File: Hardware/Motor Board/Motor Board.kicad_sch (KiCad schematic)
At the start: 14 parts, among them J1 Screw_Terminal_01x03, J2 DIN-5, J3 Conn_02x06_Counter_Clockwise, J4 Screw_Terminal_01x02, J5 Screw_Terminal_01x04, J6 Screw_Terminal_01x05, K1 SRD-24VDC-SL-C, K2 SRD-24VDC-SL-C, K3 SRD-24VDC-SL-C, K4 SRD-24VDC-SL-C

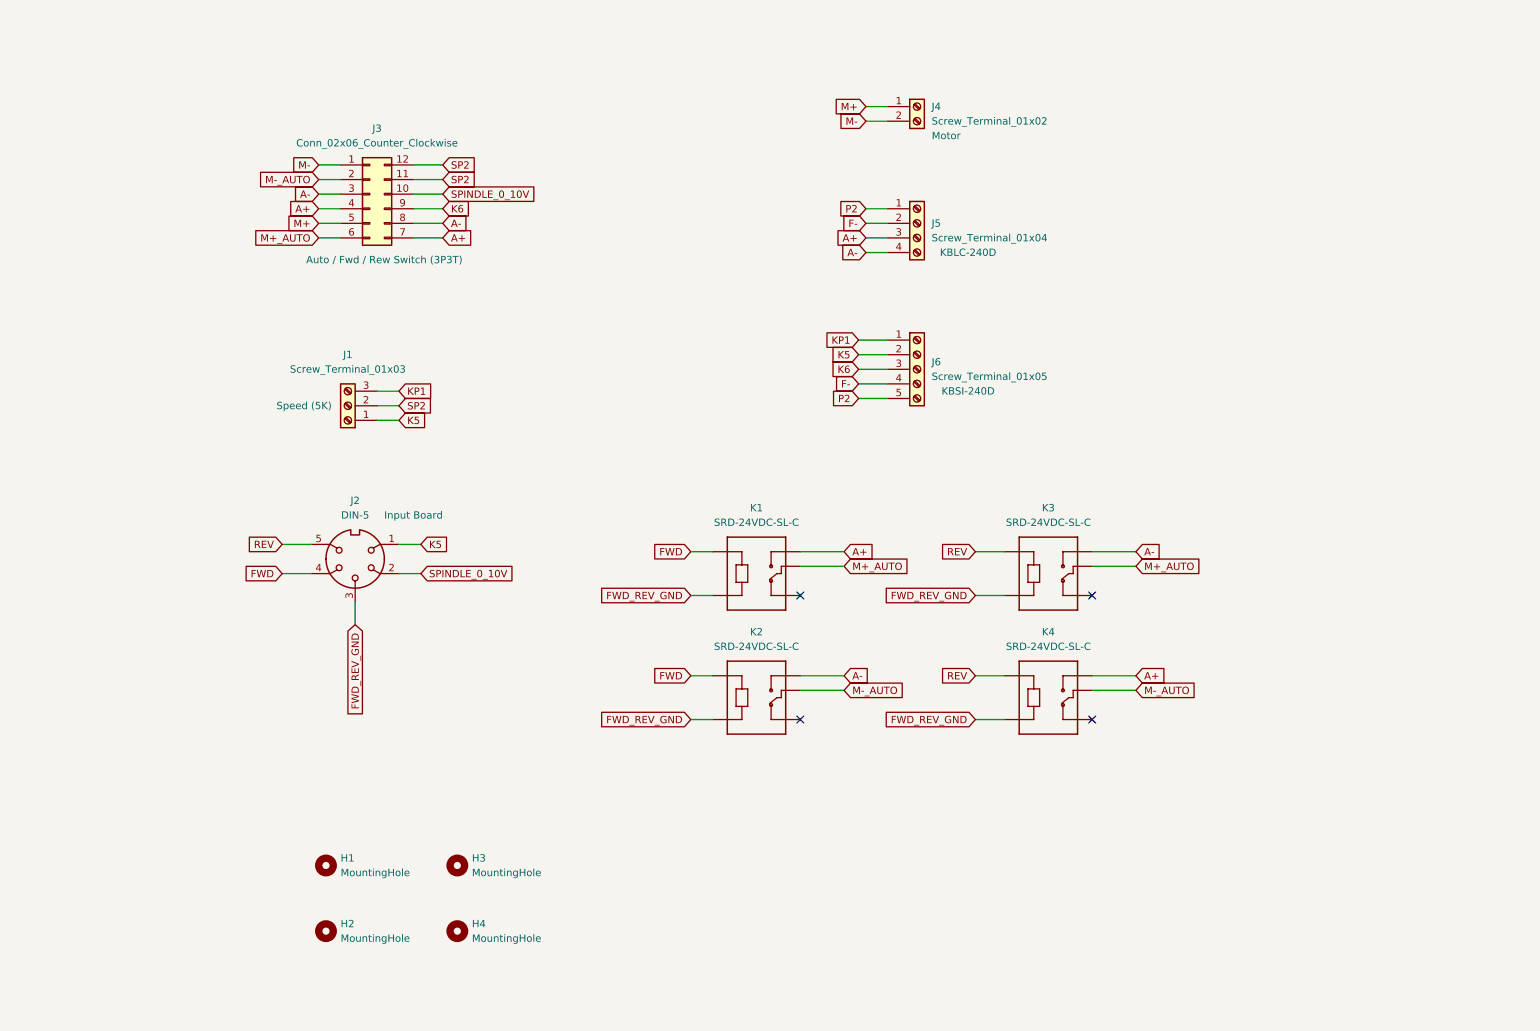
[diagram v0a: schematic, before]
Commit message: Finish schematics
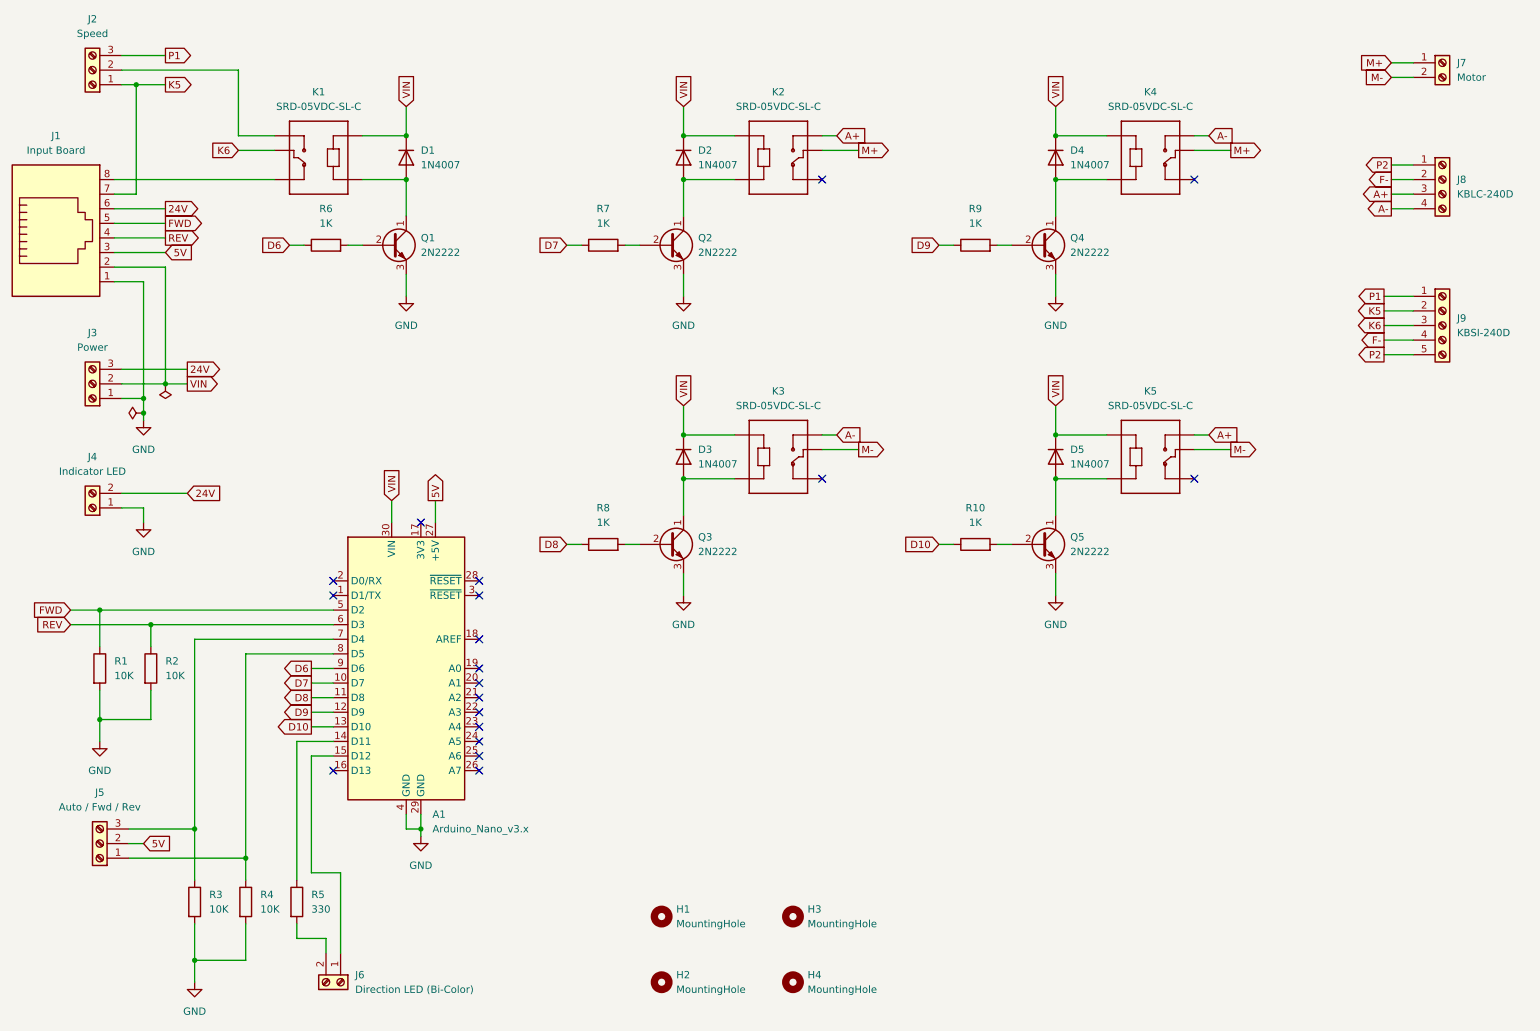
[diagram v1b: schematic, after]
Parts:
- removed J2: DIN-5, Motor Board:DIN5-RA-PTH, symbol Connector:DIN-5
- removed J3: Conn_02x06_Counter_Clockwise, Connector_Molex:Molex_Micro-Fit_3.0_43045-1200_2x06_P3.00mm_Horizontal, symbol Connector_Generic:Conn_02x06_Counter_Clockwise
- removed K1, K2, K3, K4: SRD-24VDC-SL-C, Motor Board:SRD-24VDC-SL-C, symbol SRD-24VDC-SL-C:SRD-24VDC-SL-C
- added A1: Arduino_Nano_v3.x, Module:Arduino_Nano, symbol MCU_Module:Arduino_Nano_v3.x
- added D1, D2, D3, D4, D5: 1N4007, Diode_THT:D_DO-41_SOD81_P10.16mm_Horizontal, symbol Diode:1N4007
- added J1: Input Board, Connector_RJ:RJ45_Amphenol_54602-x08_Horizontal, symbol Connector:RJ45
- added J3: Power, TerminalBlock_Phoenix:TerminalBlock_Phoenix_PT-1,5-3-5.0-H_1x03_P5.00mm_Horizontal, symbol Connector:Screw_Terminal_01x03
- added J4: Indicator LED, TerminalBlock_Phoenix:TerminalBlock_Phoenix_PT-1,5-2-5.0-H_1x02_P5.00mm_Horizontal, symbol Connector:Screw_Terminal_01x02
- added J5: Auto / Fwd / Rev, TerminalBlock_Phoenix:TerminalBlock_Phoenix_PT-1,5-3-5.0-H_1x03_P5.00mm_Horizontal, symbol Connector:Screw_Terminal_01x03
- added J6: Direction LED (Bi-Color), TerminalBlock_Phoenix:TerminalBlock_Phoenix_PT-1,5-2-5.0-H_1x02_P5.00mm_Horizontal, symbol Connector:Screw_Terminal_01x02
- added K1, K2, K3, K4, K5: SRD-05VDC-SL-C, SRD-05VDC-SL-C:SRD-05VDC-SL-C, symbol SRD05VDC-SL-C:SRD-05VDC-SL-C
- added Q1, Q2, Q3, Q4, Q5: 2N2222, Package_TO_SOT_THT:TO-92L_HandSolder, symbol Device:Q_NPN_CBE
- added R1, R2, R3, R4: 10K, Resistor_THT:R_Axial_DIN0309_L9.0mm_D3.2mm_P12.70mm_Horizontal, symbol Device:R
- added R10, R6, R7, R8, R9: 1K, Resistor_THT:R_Axial_DIN0309_L9.0mm_D3.2mm_P12.70mm_Horizontal, symbol Device:R
- added R5: 330, Resistor_THT:R_Axial_DIN0309_L9.0mm_D3.2mm_P12.70mm_Horizontal, symbol Device:R
- H1, H2, H3, H4: footprint (none) -> MountingHole:MountingHole_3.2mm_M3
- J2: renamed from J1; value Screw_Terminal_01x03 -> Speed; Label Speed (5K) -> (none)
- J7: renamed from J4; value Screw_Terminal_01x02 -> Motor; Label Motor -> (none)
- J8: renamed from J5; value Screw_Terminal_01x04 -> KBLC-240D; Label KBLC-240D -> (none)
- J9: renamed from J6; value Screw_Terminal_01x05 -> KBSI-240D; Label KBSI-240D -> (none)
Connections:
- net A+: now also K2.NO, K5.NO
- net A-: now also K3.NO, K4.NO
- net FWD: now also A1.5 (D2), J1.5, R1.1
- net K5: now also J1.7
- net K6: now also K1.COM
- net M+: now also K2.COM, K4.COM
- net M-: now also K3.COM, K5.COM
- net REV: now also A1.6 (D3), J1.4, R2.1
- net KP1 renamed P1
- net SP2: no longer names the net of J2.2 (Pin_2)
- net SP2: now also K1.NO
- new net: D2.2 (A), K2.A2, Q2.1 (C)
- new net: A1.14 (D11), R5.1
- new net: J6.2 (Pin_2), R5.2
- new net: D3.2 (A), K3.A2, Q3.1 (C)
- new net: Q3.2 (B), R8.2
- new net: D5.2 (A), K5.A2, Q5.1 (C)
- new net: A1.8 (D5), J5.1 (Pin_1), R4.1
- new net: D1.2 (A), K1.A2, Q1.1 (C)
- new net: A1.7 (D4), J5.3 (Pin_3), R3.1
- new net: Q2.2 (B), R7.2
- new net: J1.8, K1.NC
- new net: D4.2 (A), K4.A2, Q4.1 (C)
- new net: Q5.2 (B), R10.2
- new net: A1.15 (D12), J6.1 (Pin_1)
- new net: Q1.2 (B), R6.2
- new net: Q4.2 (B), R9.2
- new net 24V: J1.6, J3.3 (Pin_3), J4.2 (Pin_2)
- new net 5V: A1.27 (+5V), J1.3, J5.2 (Pin_2)
- new net D10: A1.13 (D10), R10.1
- new net D6: A1.9 (D6), R6.1
- new net D7: A1.10 (D7), R7.1
- new net D8: A1.11 (D8), R8.1
- new net D9: A1.12 (D9), R9.1
- new net GND: A1.29 (GND), A1.4 (GND), J1.1, J3.1 (Pin_1), J4.1 (Pin_1), Q1.3 (E), Q2.3 (E), Q3.3 (E), Q4.3 (E), Q5.3 (E), R1.2, R2.2, R3.2, R4.2
- new net VIN: A1.30 (VIN), D1.1 (K), D2.1 (K), D3.1 (K), D4.1 (K), D5.1 (K), J1.2, J3.2 (Pin_2), K1.A1, K2.A1, K3.A1, K4.A1, K5.A1
- no-connect marks 4 -> 19
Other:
- moved on the sheet: H1, H2, H3, H4, J2, J7, J8, J9
